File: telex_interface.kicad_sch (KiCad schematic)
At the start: 53 parts, among them J1 DB25_Female_MountingHoles, J2 Conn_02x20_Odd_Even, U1 max3387, U2 74LVC1G08

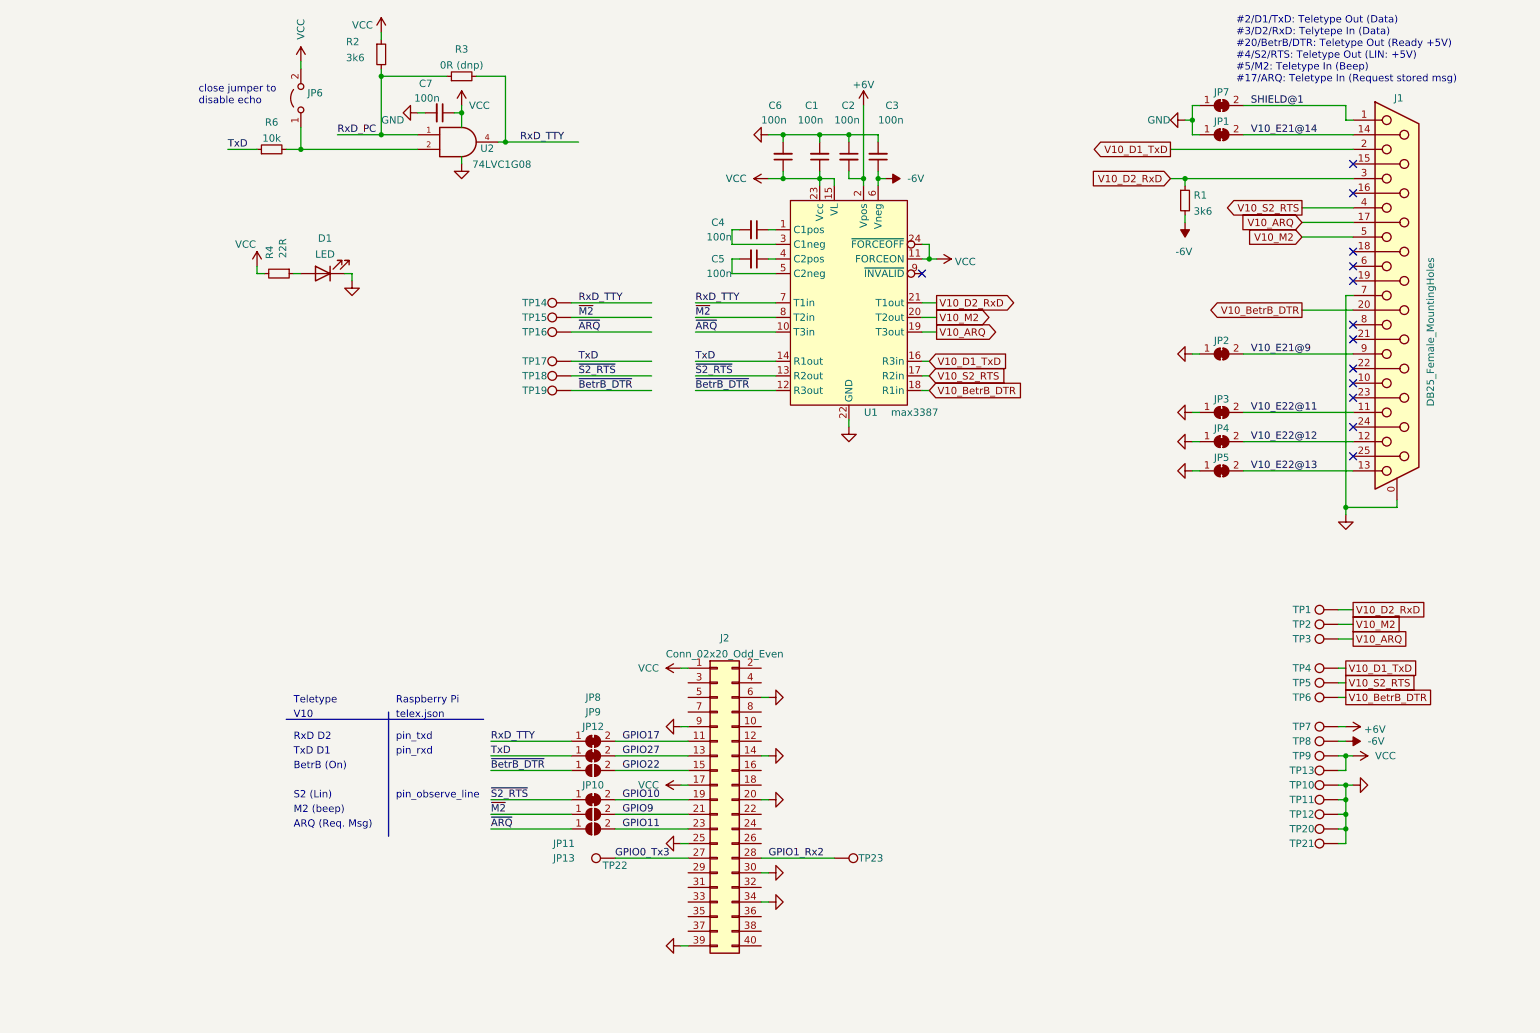
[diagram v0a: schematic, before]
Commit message: Further work...
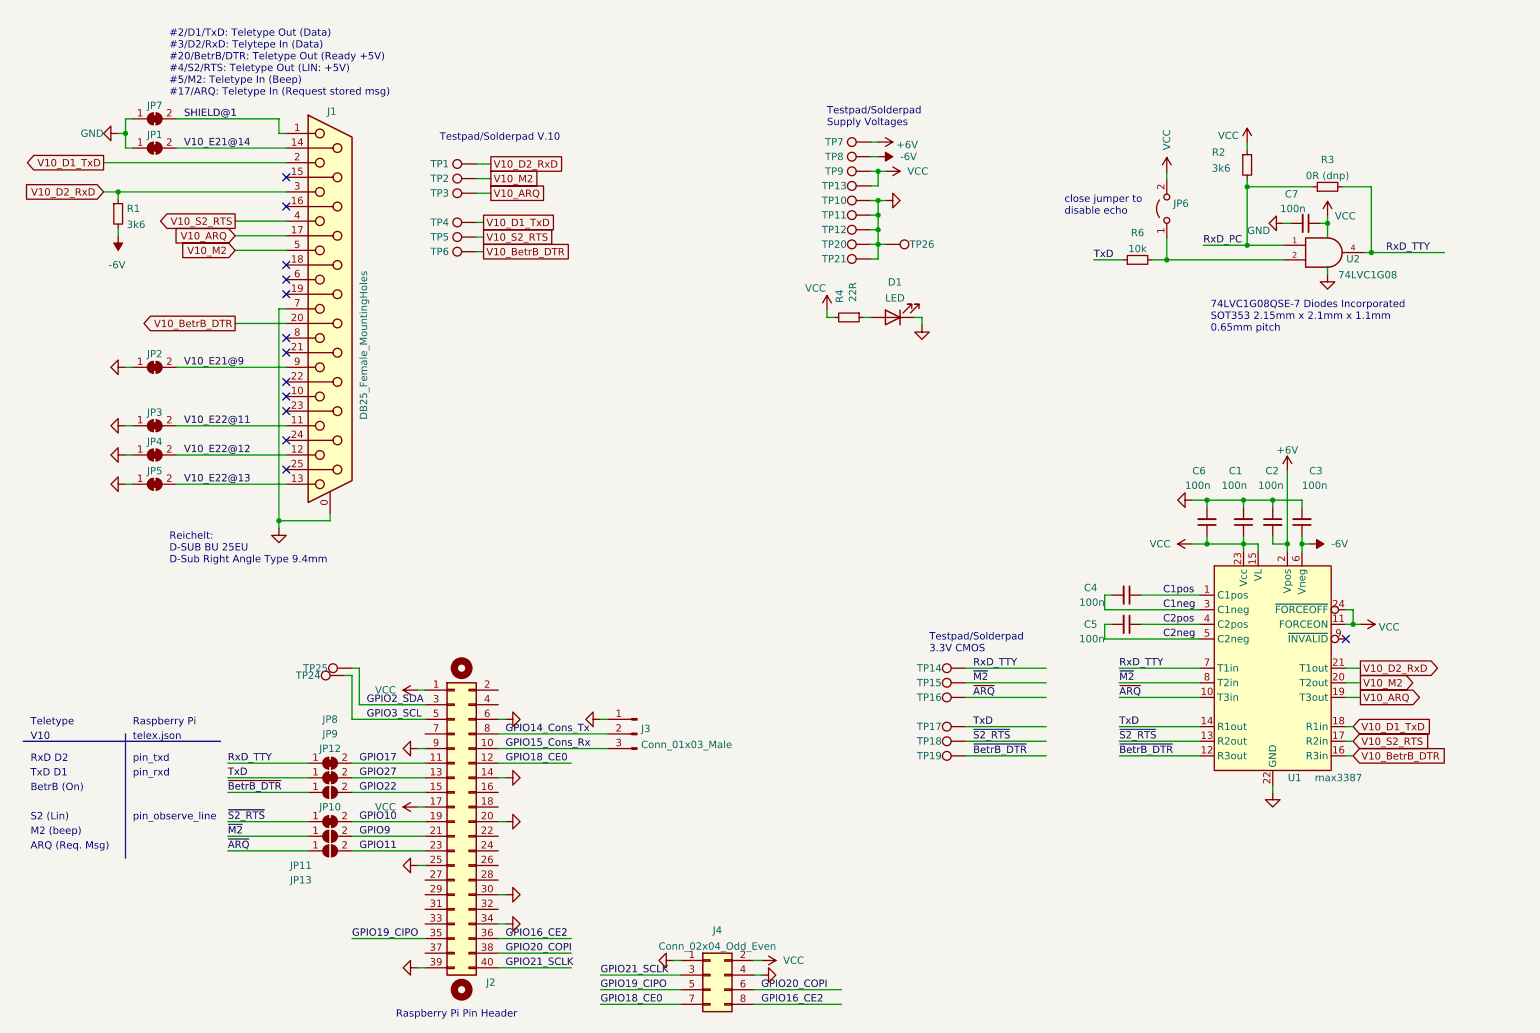
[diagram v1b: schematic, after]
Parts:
- removed TP22, TP23: TestPoint, TestPoint:TestPoint_Pad_2.0x2.0mm, symbol Connector:TestPoint
- added H1, H2: MountingHole, MountingHole:MountingHole_2.7mm_M2.5, symbol Mechanical:MountingHole
- added J3: Conn_01x03_Male, Connector_PinHeader_2.54mm:PinHeader_1x03_P2.54mm_Vertical, symbol Connector:Conn_01x03_Male
- added J4: Conn_02x04_Odd_Even, Connector_PinHeader_2.54mm:PinHeader_2x04_P2.54mm_Vertical, symbol Connector_Generic:Conn_02x04_Odd_Even
- added TP24, TP25, TP26: TestPoint, TestPoint:TestPoint_Pad_2.0x2.0mm, symbol Connector:TestPoint
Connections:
- net GND: now also J3.1 (Pin_1), J4.1 (Pin_1), J4.4 (Pin_4), TP26.1
- net V10_BetrB_DTR: now also U1.16 (R3in); no longer U1.18 (R1in)
- net V10_D1_TxD: now also U1.18 (R1in); no longer U1.16 (R3in)
- net VCC: now also J4.2 (Pin_2)
- net C1pos: now reaches C4.1, U1.1 (C1pos)
- net C1neg: now reaches C4.2, U1.3 (C1neg)
- net C2pos: now reaches C5.1, U1.4 (C2pos)
- net C2neg: now reaches C5.2, U1.5 (C2neg)
- net GPIO15_Cons_Rx: now reaches J2.10 (Pin_10)
- net GPIO15_Cons_Rx: now also J3.3 (Pin_3)
- net GPIO18_CE0: now reaches J2.12 (Pin_12)
- net GPIO18_CE0: now also J4.7 (Pin_7)
- net GPIO2_SDA: now reaches J2.3 (Pin_3)
- net GPIO2_SDA: now also TP25.1
- net GPIO19_CIPO: now reaches J2.35 (Pin_35)
- net GPIO19_CIPO: now also J4.5 (Pin_5)
- net GPIO16_CE2: now reaches J2.36 (Pin_36)
- net GPIO16_CE2: now also J4.8 (Pin_8)
- net GPIO20_COPI: now reaches J2.38 (Pin_38)
- net GPIO20_COPI: now also J4.6 (Pin_6)
- net GPIO21_SCLK: now reaches J2.40 (Pin_40)
- net GPIO21_SCLK: now also J4.3 (Pin_3)
- net GPIO3_SCL: now reaches J2.5 (Pin_5)
- net GPIO3_SCL: now also TP24.1
- net GPIO14_Cons_Tx: now reaches J2.8 (Pin_8)
- net GPIO14_Cons_Tx: now also J3.2 (Pin_2)
- net GPIO0_Tx3: no longer names the net of J2.27 (Pin_27)
- net GPIO1_Rx2: no longer names the net of J2.28 (Pin_28)
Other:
- note added: "74LVC1G08QSE-7 Diodes Incorporated SOT353 2.15mm x 2.1mm x 1.1mm 0.65mm pitch"
- note added: "Raspberry Pi Pin Header"
- note added: "Reichelt: D-SUB BU 25EU D-Sub Right Angle Type 9.4mm"
- note added: "Testpad/Solderpad 3.3V CMOS"
- note added: "Testpad/Solderpad Supply Voltages"
- note added: "Testpad/Solderpad V.10"
- moved on the sheet: C1, C2, C3, C4, C5, C6, C7, D1, J1, J2, JP1, JP10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
